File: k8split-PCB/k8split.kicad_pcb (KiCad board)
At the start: 2 copper layers, 397.3 x 124 mm, 243 parts, among them J1 AVR-ISP-6, J2 AVR-ISP-6, J3 Breakaway_Tabs, J4 Breakaway_Tabs, J5 Breakaway_Tabs, J6 Breakaway_Tabs, J7 Breakaway_Tabs, J8 Breakaway_Tabs, J9 Breakaway_Tabs, SW1 SW_Push, SW2 SW_Push, U1 ATmega32U4-AU, U2 ATmega32U4-AU, Y1 16MHz, Y2 16MHz

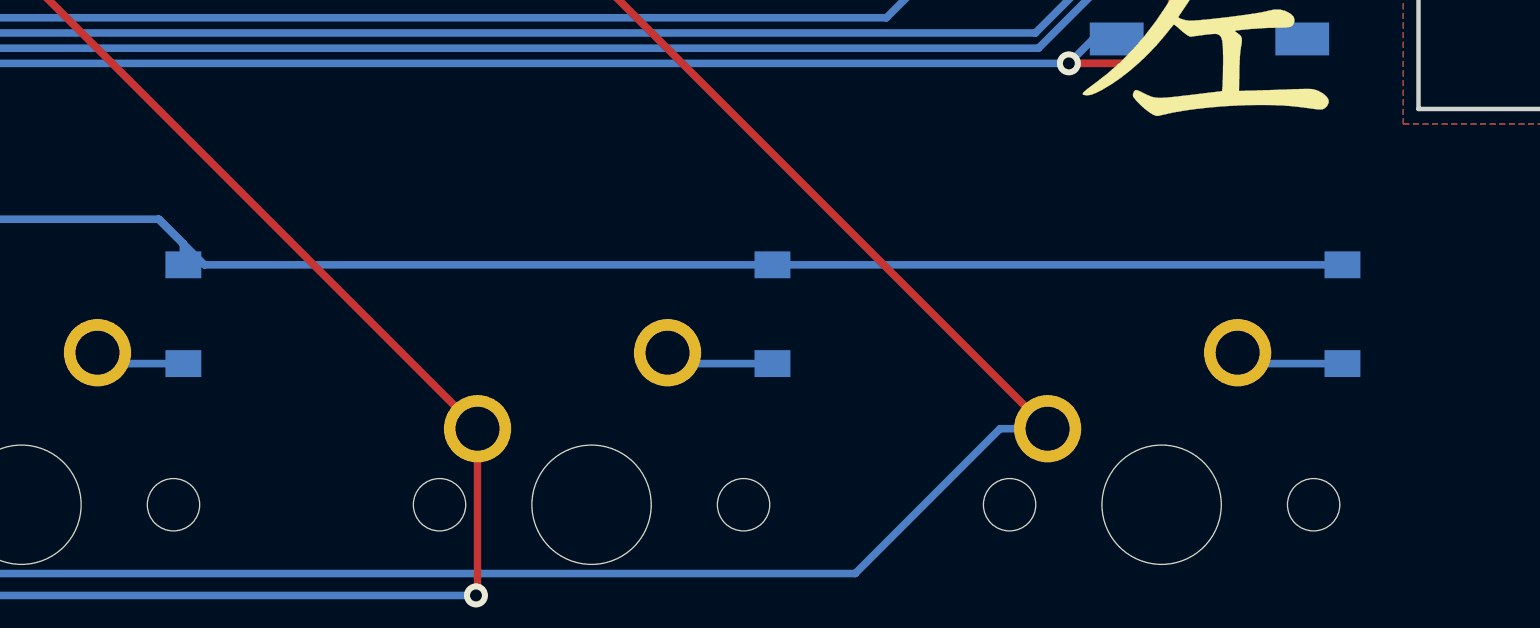
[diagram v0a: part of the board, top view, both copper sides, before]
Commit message: add some corona jokes
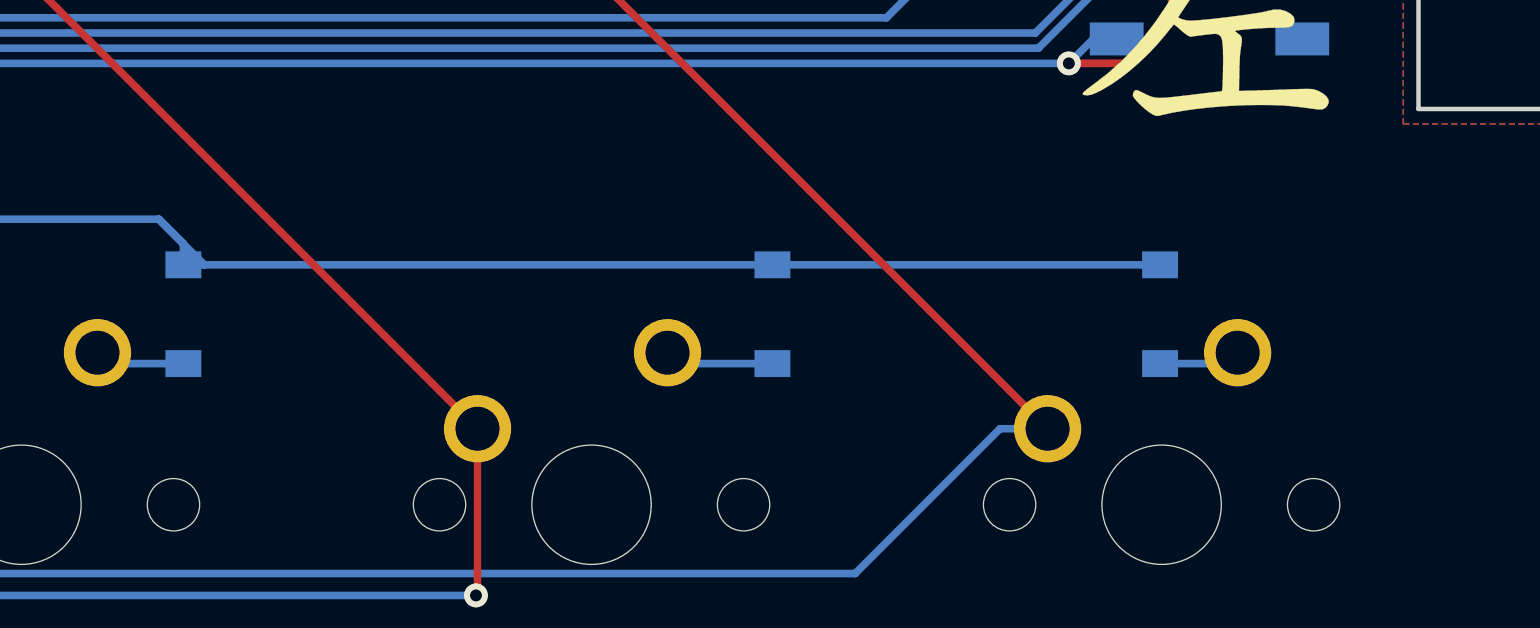
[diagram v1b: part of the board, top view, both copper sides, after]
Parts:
- added G***: LOGO, cad:corona, B.Cu at (128.5, 121.9)
- added G***: LOGO, cad:corona, B.Cu at (136.1, 121.9)
- moved D48 6.10 mm to (118.4, 125.7)
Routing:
- net ROW5: track 181.9 -> 176.5 mm
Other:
- board text added: "might contain corona proceed with caution"
